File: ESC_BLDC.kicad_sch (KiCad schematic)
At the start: 94 parts, among them J2 Conn_01x04_Pin, U10 IR2301SPBF, U11 IR2301SPBF, U4 LM339, U5 AP1509-50SG-13, U6 MCP6002-xP, U7 MCP6002-xP, U8 MCP6002-xP, U9 IR2301SPBF

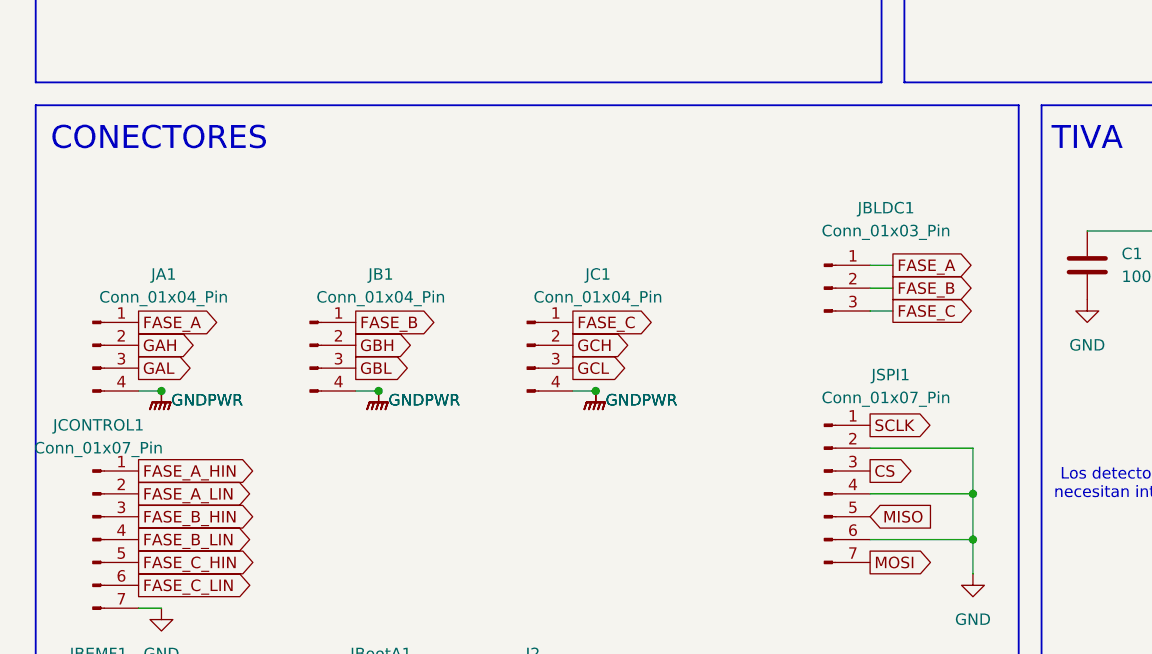
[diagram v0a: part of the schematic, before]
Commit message: routing no completo
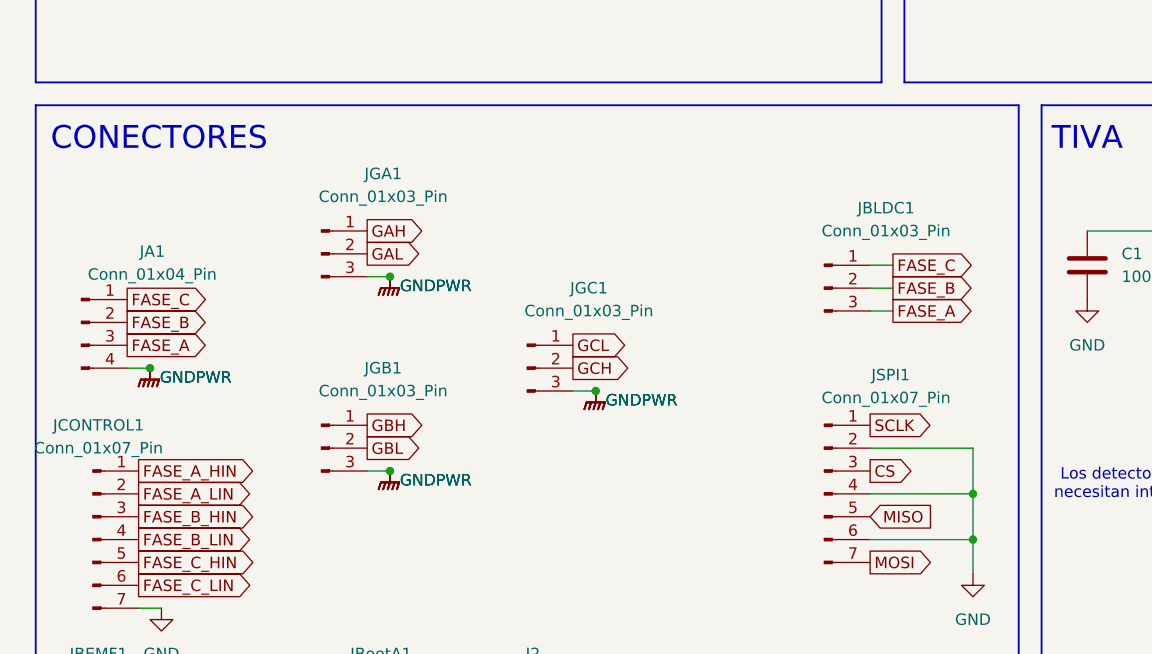
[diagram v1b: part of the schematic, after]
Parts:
- removed JB1, JC1: Conn_01x04_Pin, Connector_PinHeader_2.54mm:PinHeader_1x04_P2.54mm_Vertical, symbol Connector:Conn_01x04_Pin
- added JGA1, JGB1, JGC1: Conn_01x03_Pin, Connector_PinHeader_2.54mm:PinHeader_1x03_P2.54mm_Vertical, symbol Connector:Conn_01x03_Pin
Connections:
- net FASE_A: now also JA1.3 (Pin_3), JBLDC1.3 (Pin_3); no longer JA1.1 (Pin_1), JBLDC1.1 (Pin_1)
- net FASE_B: now also JA1.2 (Pin_2)
- net FASE_C: now also JA1.1 (Pin_1), JBLDC1.1 (Pin_1); no longer JBLDC1.3 (Pin_3)
- net GAH: now also JGA1.1 (Pin_1); no longer JA1.2 (Pin_2)
- net GAL: now also JGA1.2 (Pin_2); no longer JA1.3 (Pin_3)
- net GBH: now also JGB1.1 (Pin_1)
- net GBL: now also JGB1.2 (Pin_2)
- net GCH: now also JGC1.2 (Pin_2)
- net GCL: now also JGC1.1 (Pin_1)
- net GNDPWR: now also JGA1.3 (Pin_3), JGB1.3 (Pin_3), JGC1.3 (Pin_3)
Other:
- moved on the sheet: JA1
